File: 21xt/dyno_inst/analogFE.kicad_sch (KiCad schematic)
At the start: 80 parts, among them U12 1SS362FV_L3F, U13 1SS362FV_L3F, U14 ADA4807-2ARM, U15 ADA4807-2ARM, U16 ADA4945-1ACPZ-R2, U17 1SS362FV_L3F, U18 1SS362FV_L3F, U19 ADA4807-1, U20 ADA4807-1, U22 ADA4945-1ACPZ-R2

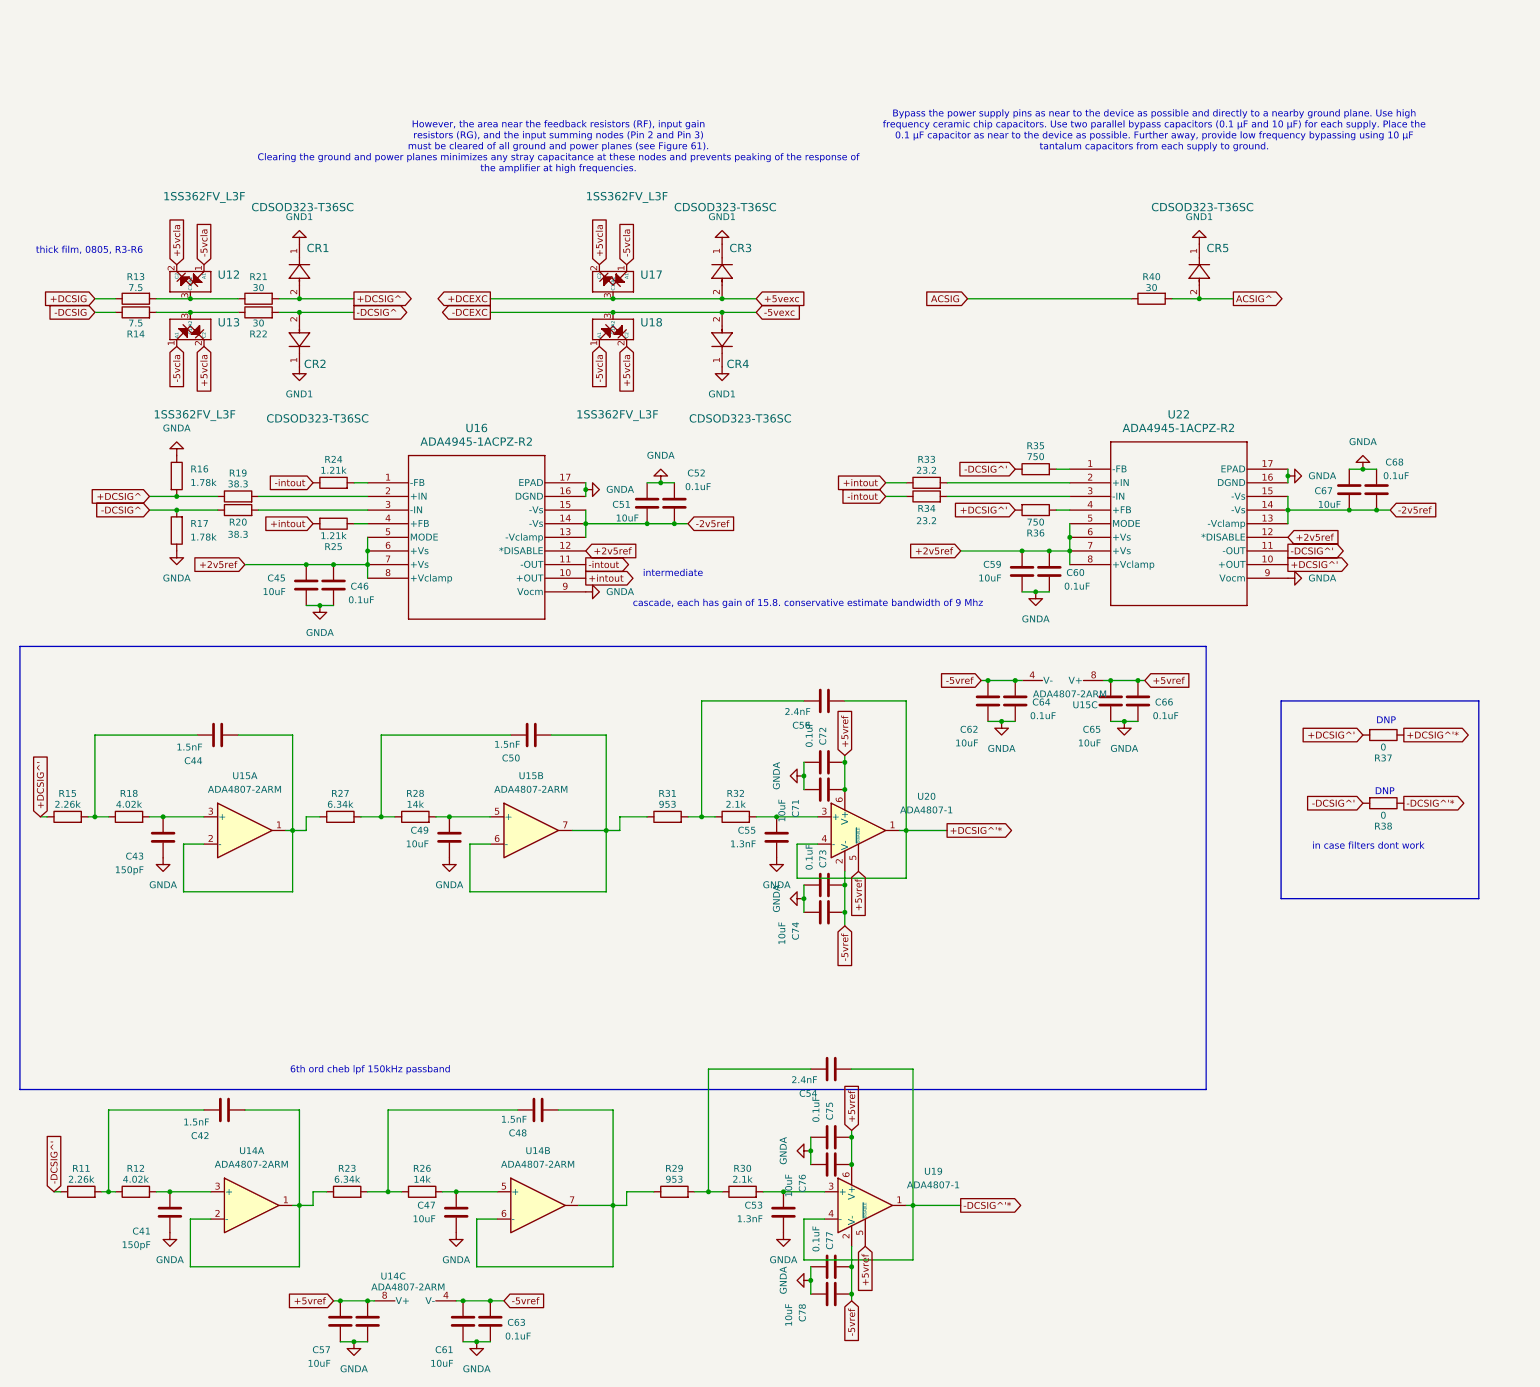
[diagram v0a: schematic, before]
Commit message: dddd
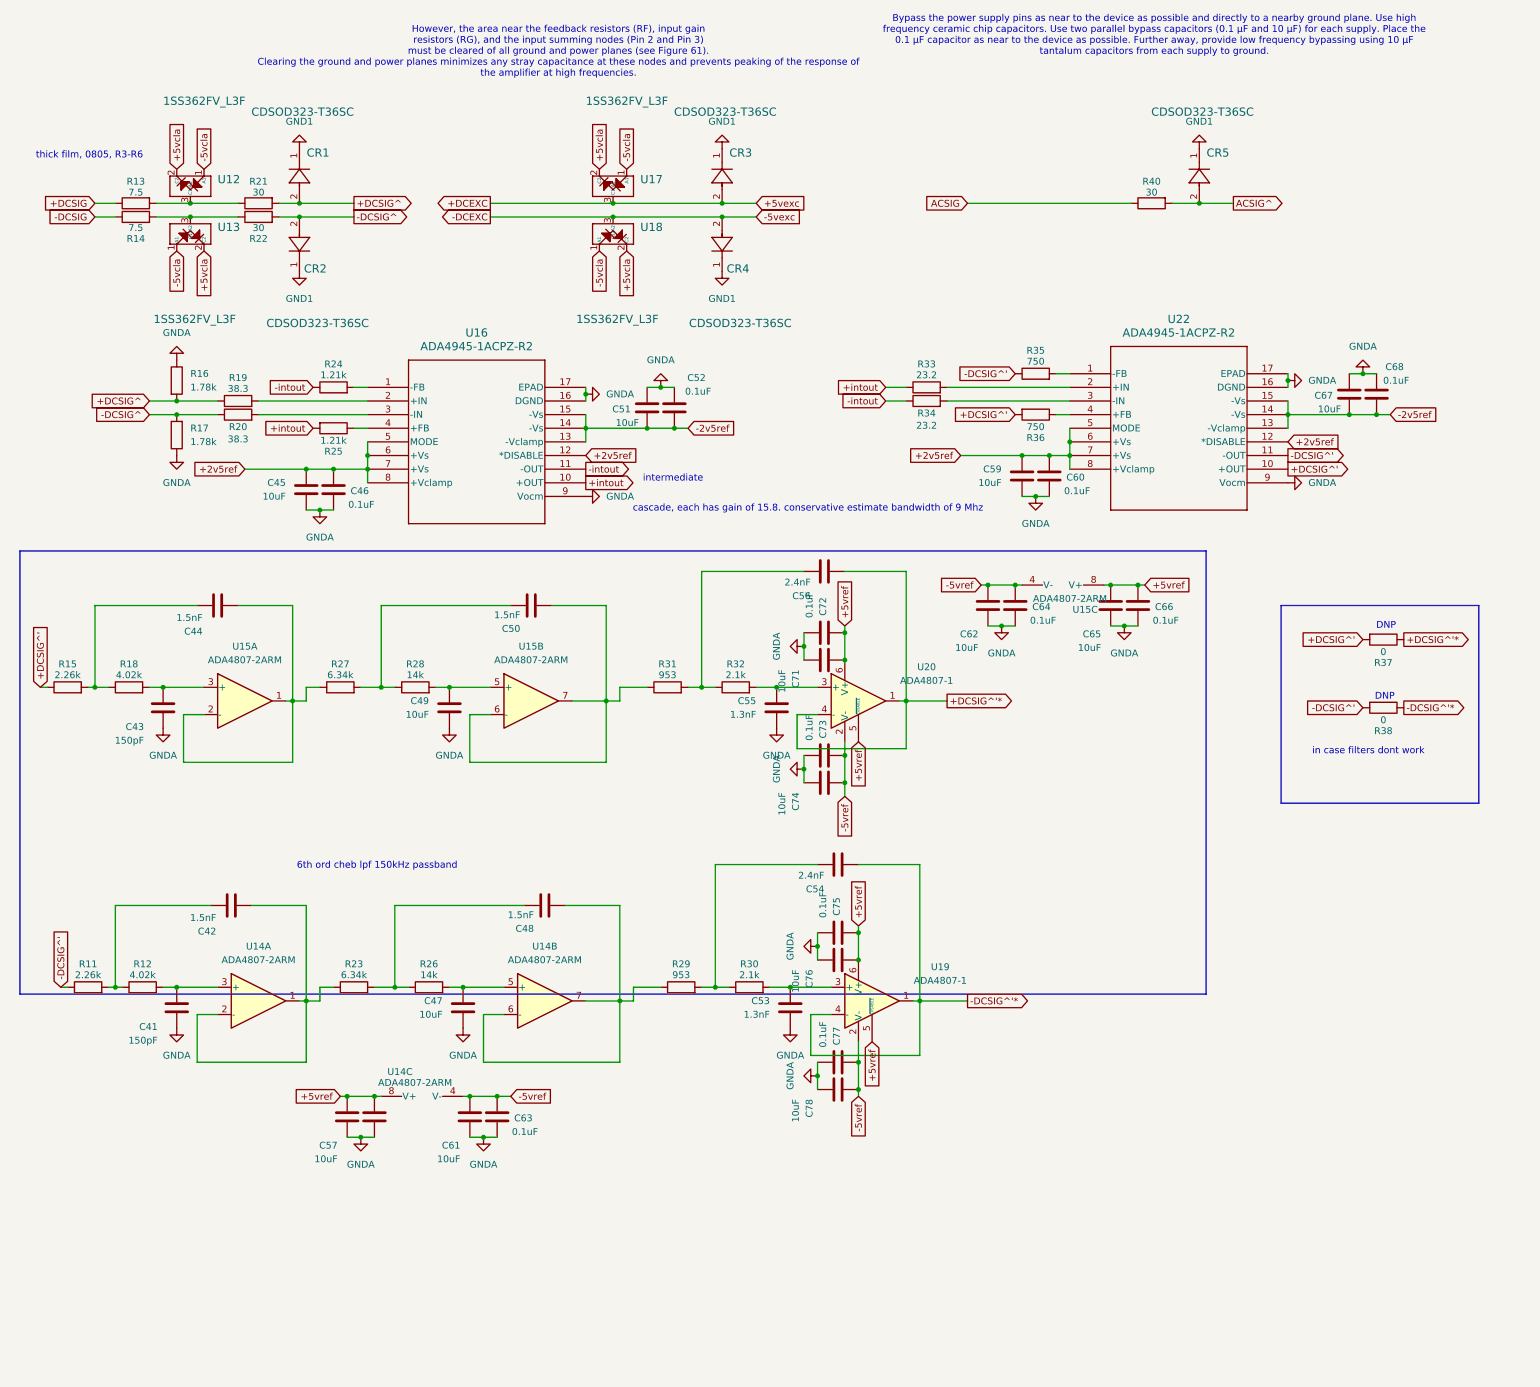
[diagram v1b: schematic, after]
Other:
- moved on the sheet: C41, C42, C43, C44, C45, C46, C47, C48, C49, C50, C51, C52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
